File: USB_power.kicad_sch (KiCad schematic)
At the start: 13 parts, among them J1 PWR_IN, J2 USB_A

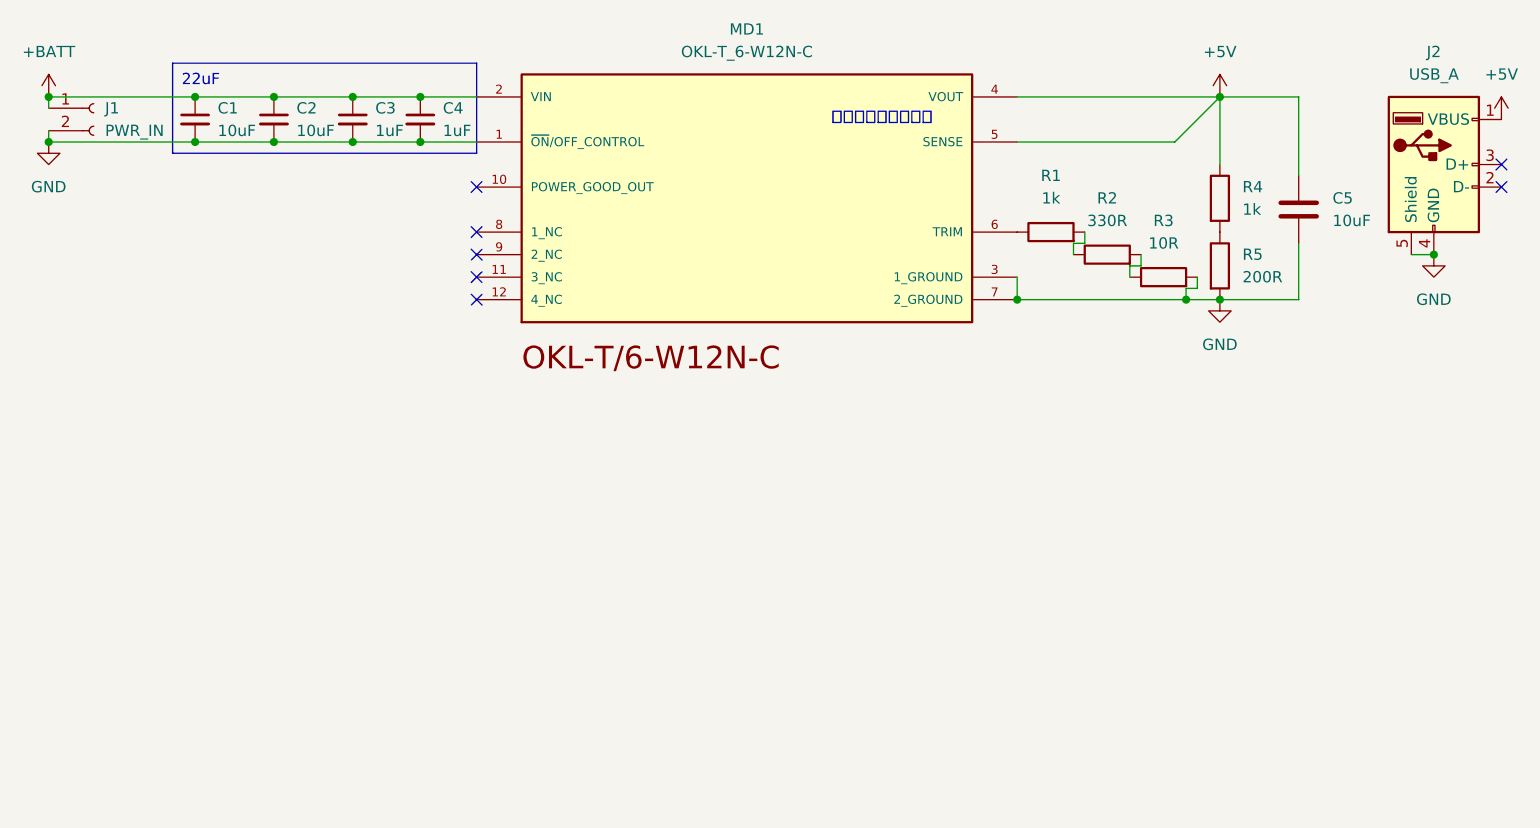
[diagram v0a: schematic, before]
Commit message: 名前変更
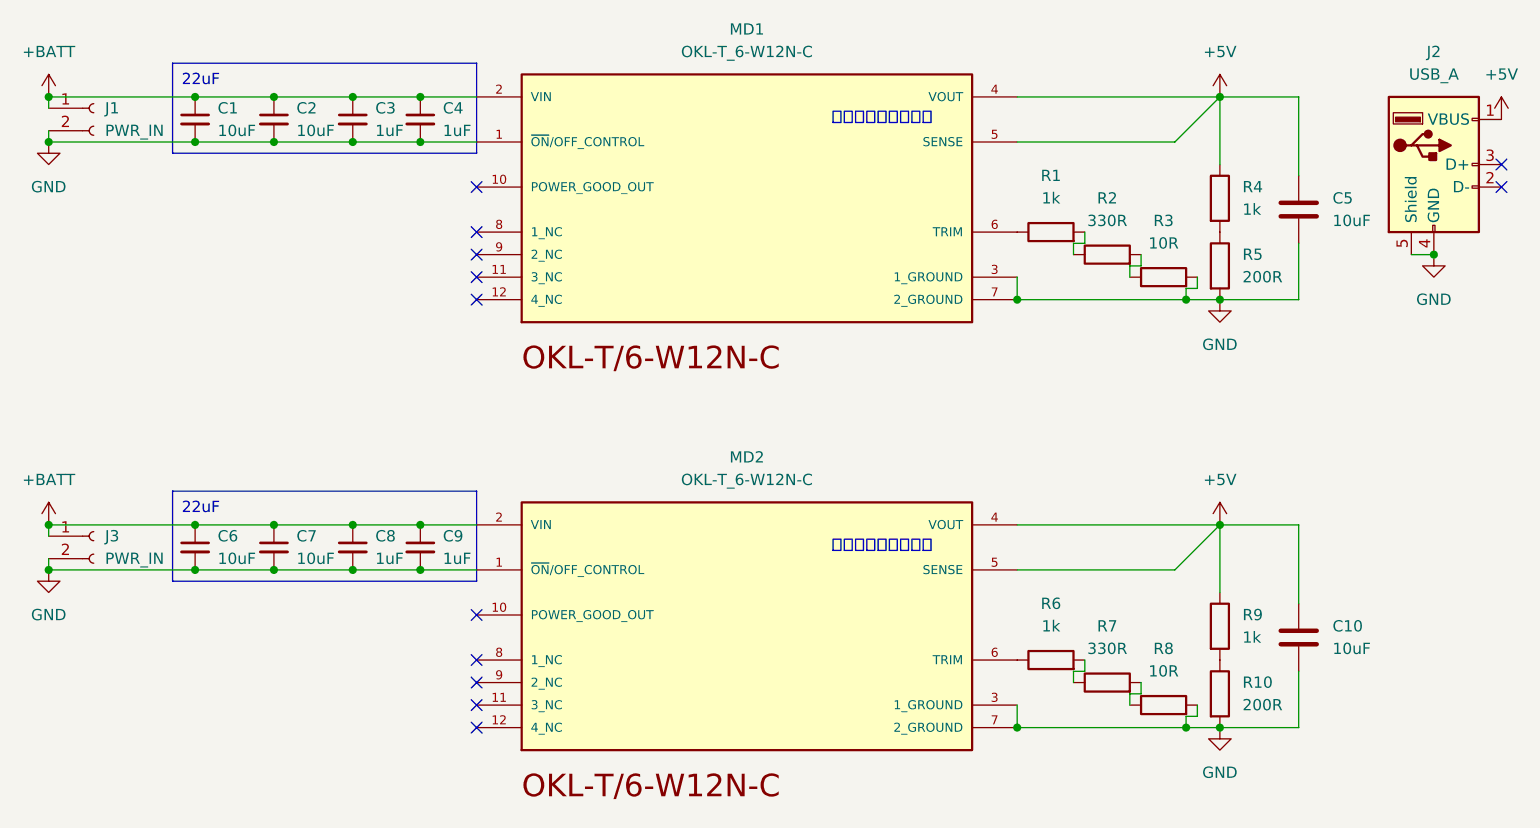
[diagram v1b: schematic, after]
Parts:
- added C10: 10uF, Capacitor_SMD:C_0805_2012Metric, symbol Device:C
- added C6, C7: 10uF, Capacitor_SMD:C_0805_2012Metric, symbol Device:C_Small
- added C8, C9: 1uF, Capacitor_SMD:C_0805_2012Metric, symbol Device:C_Small
- added J3: PWR_IN, Connector_AMASS:AMASS_XT60-M_1x02_P7.20mm_Vertical, symbol Connector:Conn_01x02_Socket
- added MD2: OKL-T_6-W12N-C, Pi_Header:MURATA_OKL-T-6-W12N-C_0, symbol OKL-T_6-W12N-C:OKL-T_6-W12N-C
- added R10: 200R, Resistor_SMD:R_0805_2012Metric, symbol Device:R
- added R6, R9: 1k, Resistor_SMD:R_0805_2012Metric, symbol Device:R
- added R7: 330R, Resistor_SMD:R_0805_2012Metric, symbol Device:R
- added R8: 10R, Resistor_SMD:R_0805_2012Metric, symbol Device:R
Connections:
- net +5V: now also C10.1, MD2.4 (VOUT), MD2.5 (SENSE), R9.1
- net +BATT: now also C6.1, C7.1, C8.1, C9.1, J3.1 (Pin_1), MD2.2 (VIN)
- net GND: now also C10.2, C6.2, C7.2, C8.2, C9.2, J3.2 (Pin_2), MD2.1 (~{ON}/OFF_CONTROL), MD2.3 (1_GROUND), MD2.7 (2_GROUND), R10.2, R8.2
- new net: R10.1, R9.2
- new net: MD2.6 (TRIM), R6.1
- new net: R7.2, R8.1
- new net: R6.2, R7.1
- no-connect marks 7 -> 12
